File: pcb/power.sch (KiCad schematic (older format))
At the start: 7 parts, among them U6 ADP2108AUJ-3.3

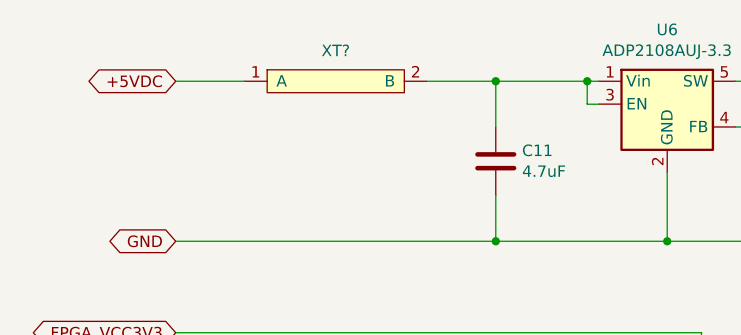
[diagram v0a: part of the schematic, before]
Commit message: more footprints assigned
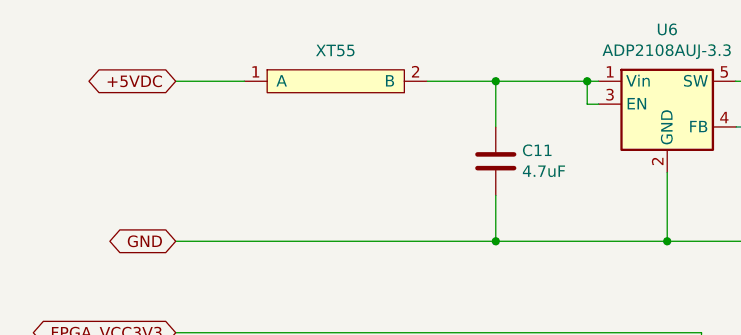
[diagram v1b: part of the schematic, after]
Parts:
- JP1: footprint (none) -> Connector_PinSocket_2.54mm:PinSocket_1x03_P2.54mm_Vertical
- JP2: footprint (none) -> Connector_PinSocket_2.54mm:PinSocket_1x02_P2.54mm_Vertical
- XT55: renamed from XT?; footprint (none) -> WM1200:testpoint_cutline
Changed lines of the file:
@@
 $EndComp
 $Comp
-L WM1200:testpoint_cutline XT?
+L WM1200:testpoint_cutline XT55
 U 1 1 5E716612
 P 2300 2050
-F 0 "XT?" H 2300 2233 50  0000 C CNN
+F 0 "XT55" H 2300 2233 50  0000 C CNN
 F 1 "testpoint_cutline" H 2300 2200 50  0001 C CNN
-F 2 "" H 2450 2050 50  0001 C CNN
+F 2 "WM1200:testpoint_cutline" H 2450 2050 50  0001 C CNN
 F 3 "" H 2450 2050 50  0001 C CNN
 	1    2300 2050
@@
 F 0 "JP1" V 3854 3602 50  0000 L CNN
 F 1 "Jumper_NC_Dual" V 3945 3602 50  0000 L CNN
-F 2 "" H 3900 3500 50  0001 C CNN
+F 2 "Connector_PinSocket_2.54mm:PinSocket_1x03_P2.54mm_Vertical" H 3900 3500 50  0001 C CNN
 F 3 "~" H 3900 3500 50  0001 C CNN
 	1    3900 3500
@@
 F 0 "JP2" H 3900 4764 50  0000 C CNN
 F 1 "Jumper" H 3900 4673 50  0000 C CNN
-F 2 "" H 3900 4500 50  0001 C CNN
+F 2 "Connector_PinSocket_2.54mm:PinSocket_1x02_P2.54mm_Vertical" H 3900 4500 50  0001 C CNN
 F 3 "~" H 3900 4500 50  0001 C CNN
 	1    3900 4500
